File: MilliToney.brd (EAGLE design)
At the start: 50 x 50 mm, 73 parts, among them J1 BANANA_CONN, J2 BANANA_CONN, J3 BNCPTH, Q1 BC807-16LT1SMD, U1 NCP303LSN09, U2 TLV431BIDBZR, U3 OPA335AIDBVT, U4 MCP6001T-E/OT, U5 Comparator

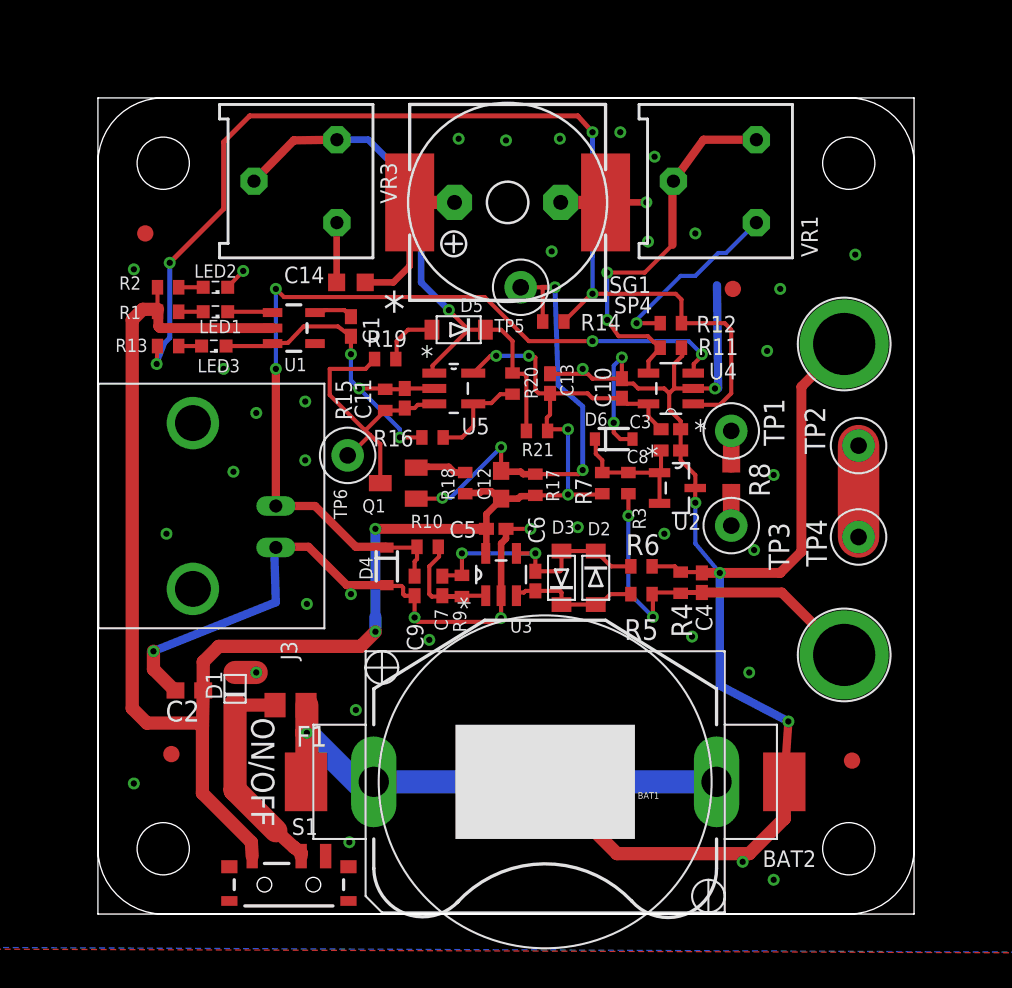
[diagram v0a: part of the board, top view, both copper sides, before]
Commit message: Minor updates
Minor Updates
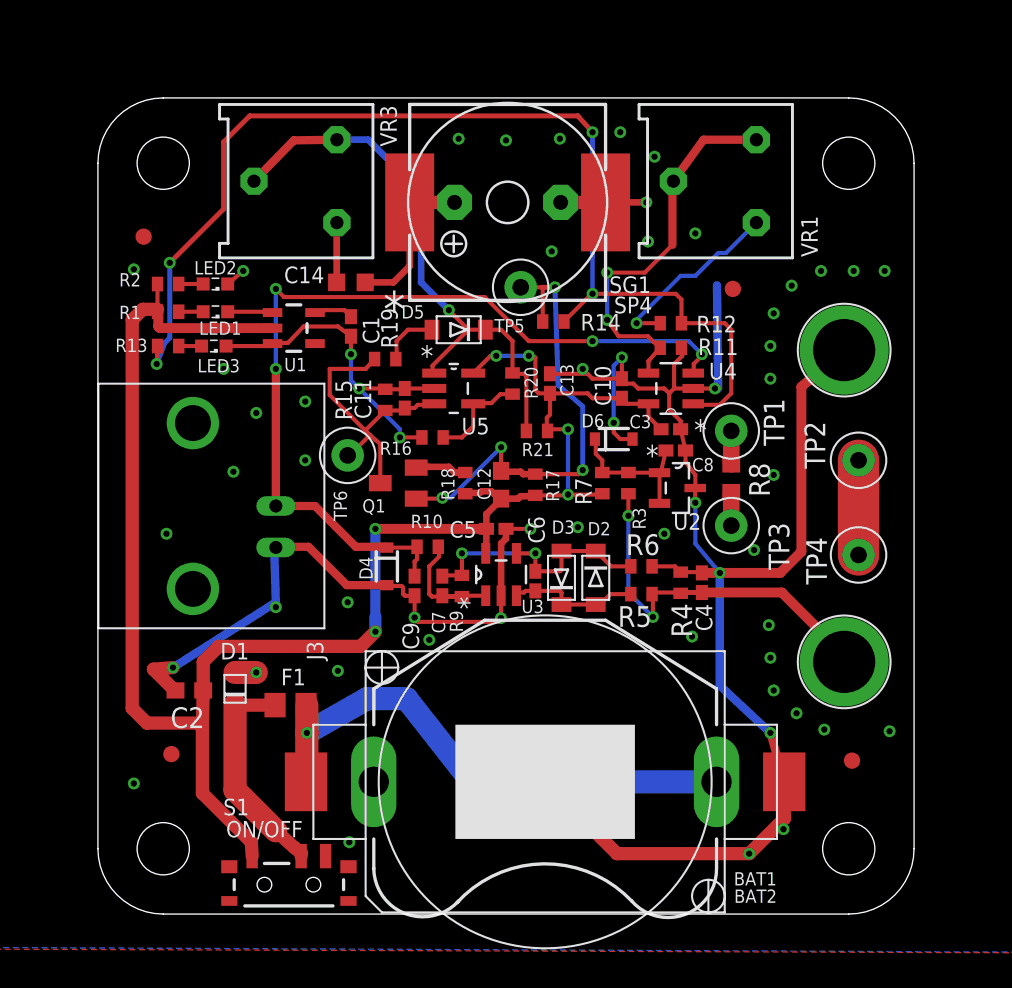
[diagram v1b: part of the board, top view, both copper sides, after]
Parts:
- moved TP4 1.10 mm to (46.6, 22.0)
- moved TP2 0.90 mm to (46.6, 27.8)
- moved J2 0.43 mm to (45.7, 15.4)
- moved LOGO1 0.40 mm to (26.6, 16.1)
- moved J1 0.38 mm to (45.7, 34.5)
- moved C8 0.30 mm to (35.4, 28.4)
- moved U$3 0.22 mm to (2.80, 41.5)
- moved LED2 0.20 mm to (7.20, 38.6)
- moved R2 0.20 mm to (4.30, 38.6)
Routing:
- net GND: track 168.3 -> 166.6 mm, vias 49 -> 58
- net N$1: track 31.2 -> 32.9 mm
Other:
- outline, holes or cut-outs redrawn
- board text added: "MilliToney"
- board text removed: "MicroToney"
